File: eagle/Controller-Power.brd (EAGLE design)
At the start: 71 x 64 mm, 24 parts, among them IC3 7818TV, X1 MKDSN1,5/2-5,08, X2 MKDSN1,5/2-5,08, X3 MKDSN1,5/2-5,08

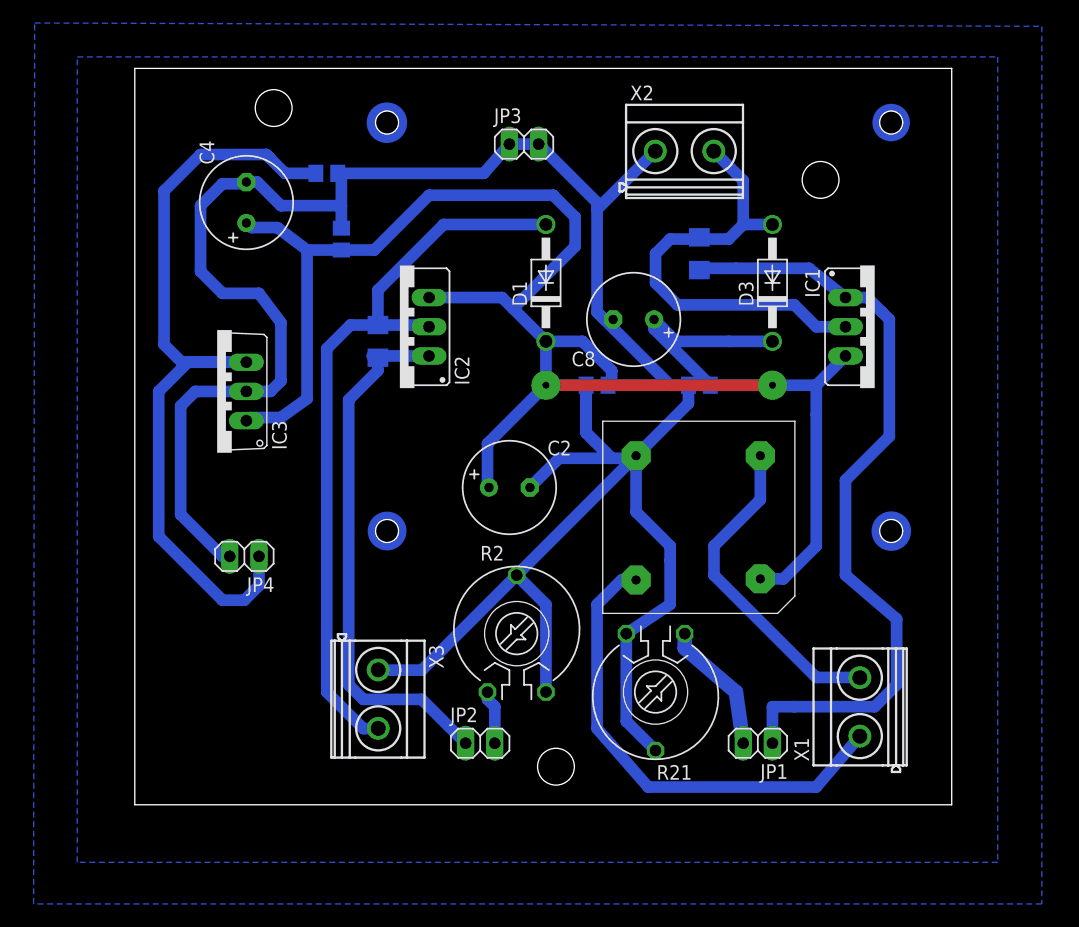
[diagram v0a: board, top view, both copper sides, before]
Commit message: Lots of schema and board changes
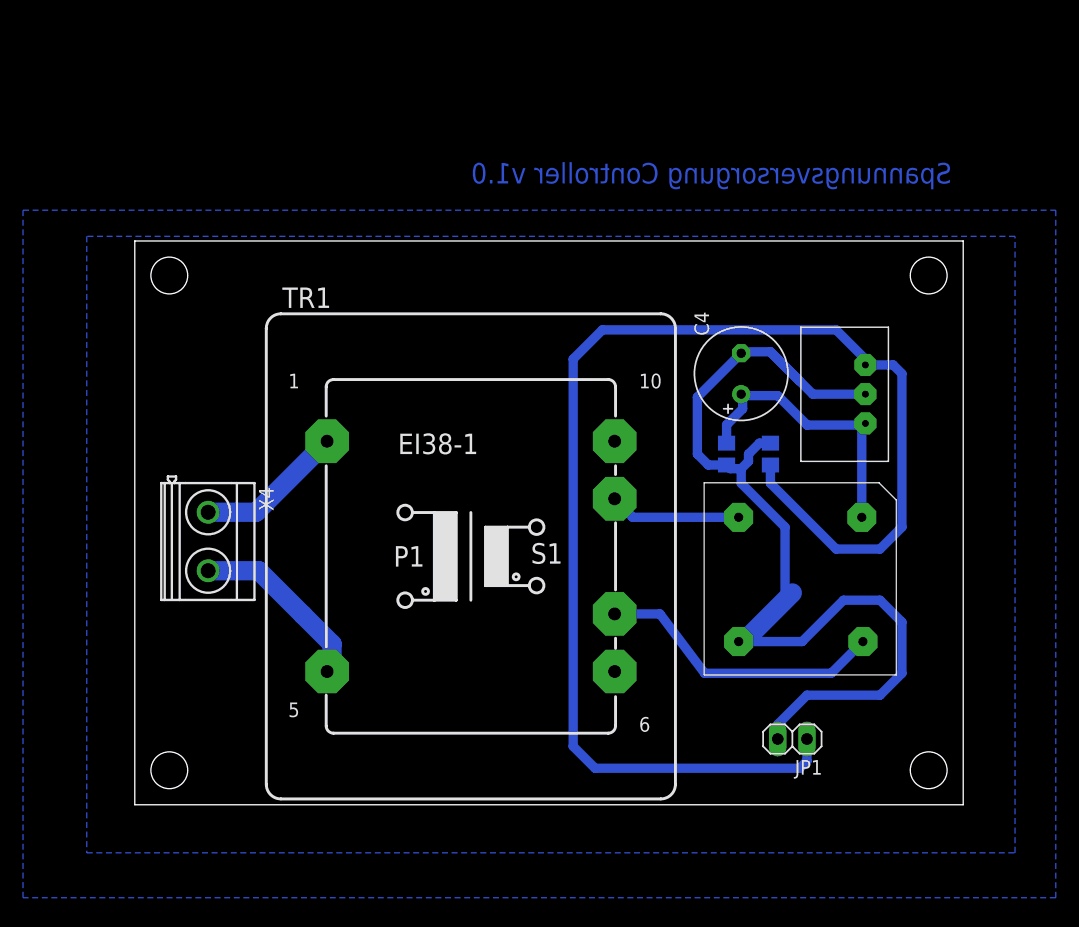
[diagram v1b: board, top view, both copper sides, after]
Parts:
- removed C1, C7: 100nF, rcl:C0805
- removed C2, C8: 100µ, rcl:E3,5-8
- removed D1, D3: 1N4004, diode:DO41-10
- removed IC1: (no value), v-reg:317TS
- removed IC3: 7818TV, linear:TO220V
- removed JP2, JP3, JP4: (no value), pinhead:1X02
- removed R1, R20: 100k, rcl:R1206
- removed R2, R21: (no value), pot:PT-10
- removed U$2: GLEICHRICHTER, Gleichrichter:KBPC1
- removed X1, X2, X3: MKDSN1,5/2-5,08, con-phoenix-508:MKDSN1,5/2-5,08
- added TR1: (no value), trafo:EI38-1
- added U$1: GLEICHRICHTER, Gleichrichter:KBPC1
- added X4: MKDSN1,5/2-5,08, con-phoenix-508:MKDSN1,5/2-5,08
- IC2: value (none) -> DCDC-WANDLER; device v-reg:317TS -> 0liver:TRACOPOWER-DCDCWANDER-TSR1
- moved C6 45.6 mm to (55.2, 30.5), turned to 90 degrees
- moved C4 45.5 mm to (52.7, 37.5)
- moved IC2 41.3 mm to (63.5, 33.1)
- moved C5 38.3 mm to (51.4, 30.5), turned to 270 degrees
- moved JP1 3.02 mm to (57.1, 5.71)
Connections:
- removed net N$2: C6.1, IC3.3, JP4.1
- removed net N$24: U$2.AC1, X1.2
- removed net N$28: D3.A, IC1.2, R20.2, X2.2
- removed net N$29: JP1.2, R21.A
- removed net N$3: D1.A, IC2.2, R1.2, X3.2
- removed net N$30: IC1.1, JP1.1, R20.1
- removed net N$4: IC2.1, JP2.1, R1.1
- removed net N$5: JP2.2, R2.A
- new net N$19: TR1.1, X4.1
- new net N$20: TR1.5, X4.2
- new net N$21: TR1.7, U$1.AC2
- new net N$22: TR1.9, U$1.AC1
- net GND: now also IC2.2, JP1.2, U$1.-; no longer C1.2, C2.-, C7.2, C8.-, IC3.2, JP3.1, JP3.2, JP4.2, R2.E, R2.S, R21.E, R21.S, U$2.-, X2.1, X3.1
- net N$17: now also IC2.1, U$1.+; no longer C1.1, C2.+, C7.1, C8.+, D1.C, D3.C, IC1.3, IC2.3, IC3.1, U$2.+
- net N$25: now also C6.1, IC2.3, JP1.1; no longer U$2.AC2, X1.1
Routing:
- net N$17: track 172.6 -> 25.4 mm, vias 2 -> 0
- net GND: track 222.4 -> 94.0 mm
- net N$25: track 42.2 -> 118.2 mm
- net N$2: track 72.1 -> 0.00 mm
- net N$30: track 68.5 -> 0.00 mm
- net N$3: track 65.4 -> 0.00 mm
- net N$4: track 47.2 -> 0.00 mm
- net N$28: track 39.4 -> 0.00 mm
- net N$24: track 28.4 -> 0.00 mm
- net N$21: track 0.00 -> 25.3 mm
- net N$20: track 0.00 -> 18.2 mm
- net N$19: track 0.00 -> 12.9 mm
- net N$29: track 11.6 -> 0.00 mm
- net N$22: track 0.00 -> 11.5 mm
- net N$5: track 4.71 -> 0.00 mm
- added copper zone on layer 16, net N$16
- removed copper zone on layer 16, net N$1
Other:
- board size 71 x 64 mm -> 72 x 49 mm
- board text added: "Spannungsversorgung Controller v1.0"
- board text removed: "36V ~ IN"
- board text removed: "GND"
- board text removed: "Poti V1"
- board text removed: "Poti V2"
- board text removed: "Widerstandskaskade 1"
- board text removed: "Widerstandskaskade 2"
